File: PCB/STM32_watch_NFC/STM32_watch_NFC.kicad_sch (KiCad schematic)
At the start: 60 parts, among them J1 Conn_01x06_Socket, Q1 2N7000, SW1 SW_DPST_x2, SW2 SW_DPST_x2, SW3 SW_DPST_x2, U1 STM32L031G6Ux, Y2 32.768kHz

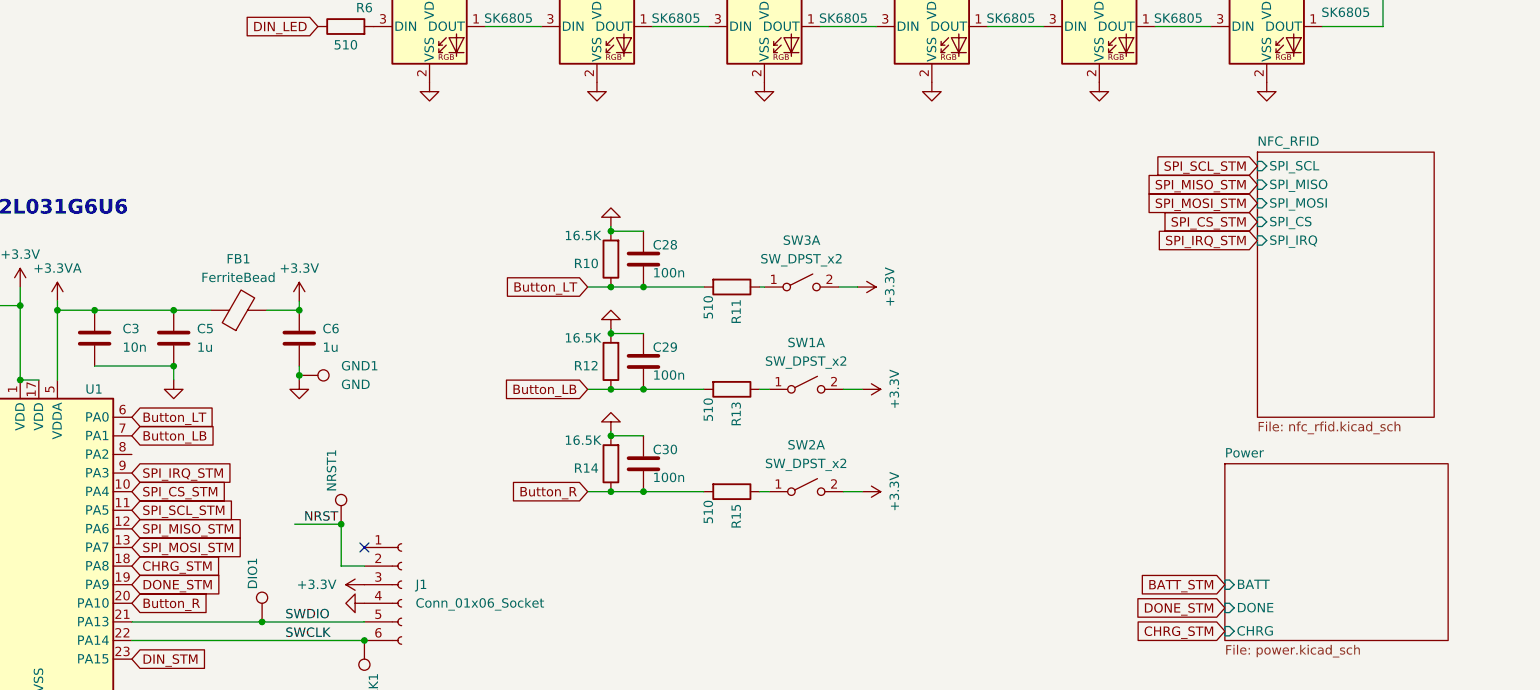
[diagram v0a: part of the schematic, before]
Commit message: new branch
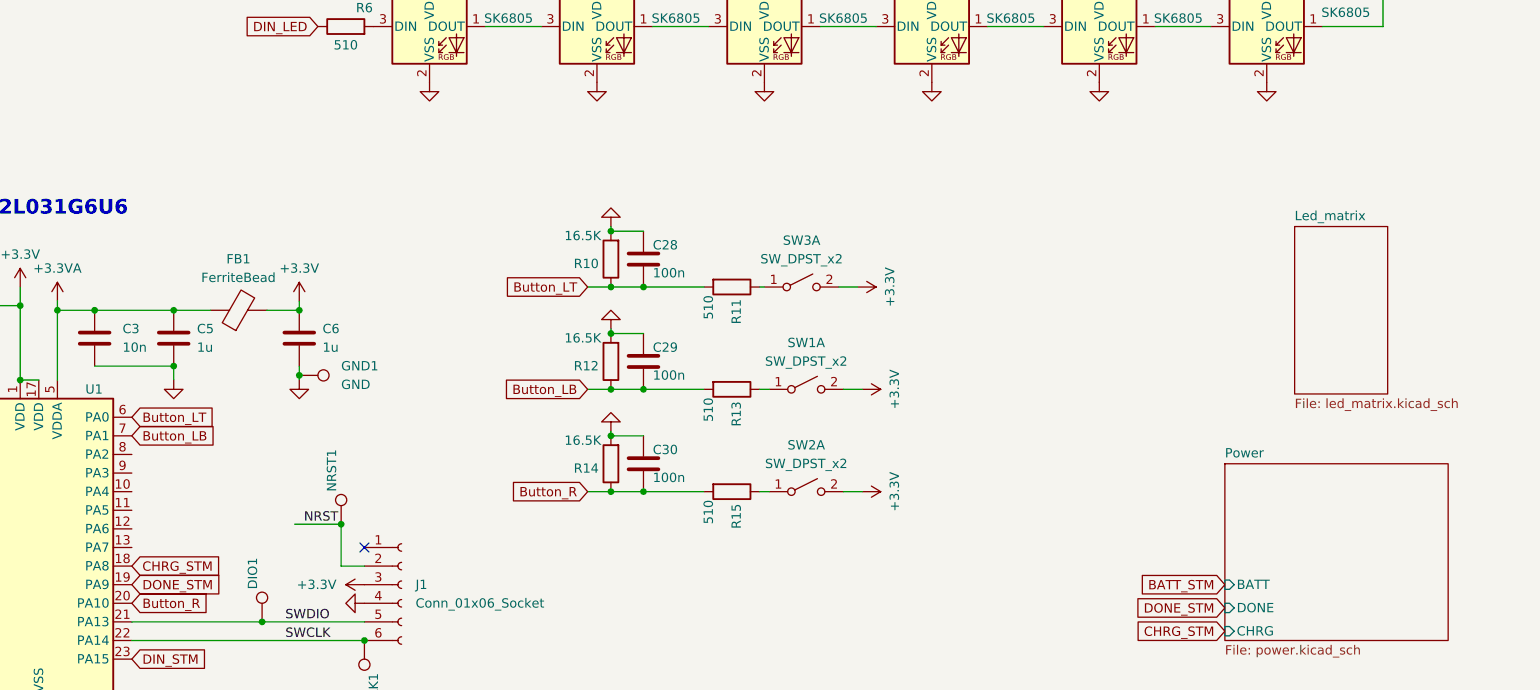
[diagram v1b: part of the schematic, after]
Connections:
- net SPI_CS_STM: no longer names the net of U1.10 (PA4)
- net SPI_IRQ_STM: no longer names the net of U1.9 (PA3)
- net SPI_MISO_STM: no longer names the net of U1.12 (PA6)
- net SPI_MOSI_STM: no longer names the net of U1.13 (PA7)
- net SPI_SCL_STM: no longer names the net of U1.11 (PA5)
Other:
- removed sheet NFC_RFID
- added sheet Led_matrix (led_matrix.kicad_sch)
